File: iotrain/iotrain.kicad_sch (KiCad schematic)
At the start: 69 parts, among them J1 12V, J10 X2, J11 SCL, J12 SDA, J13 GND, J14 3V3, J15 GND, J16 USB_B_Micro, J2 PROG ESP, J3 AC1, J4 AC1, J5 LSP, J6 LSP, J7 M1, J8 M2, J9 X1, Q1 TPM2008 EP3-A, Q2 TPM2008 EP3-A, SW1 Reset, SW2 Boot, U2 MAX98357A_WLP_Package, U3 TPS82130, U4 ESP32-C6FH4, U6 IPS_160_40_10P, U7 DRV8876RGT, Y1 40MHz

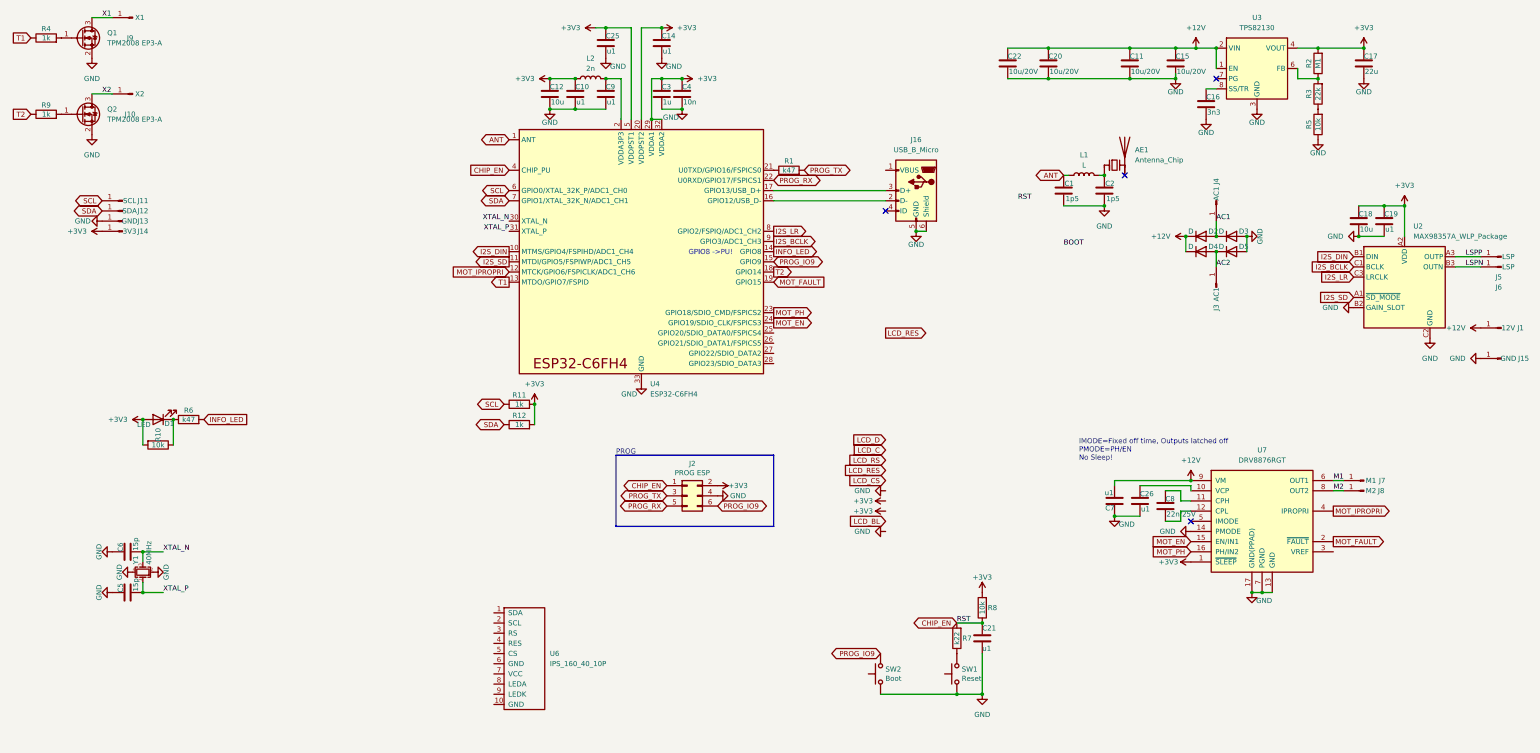
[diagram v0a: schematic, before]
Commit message: Beautified
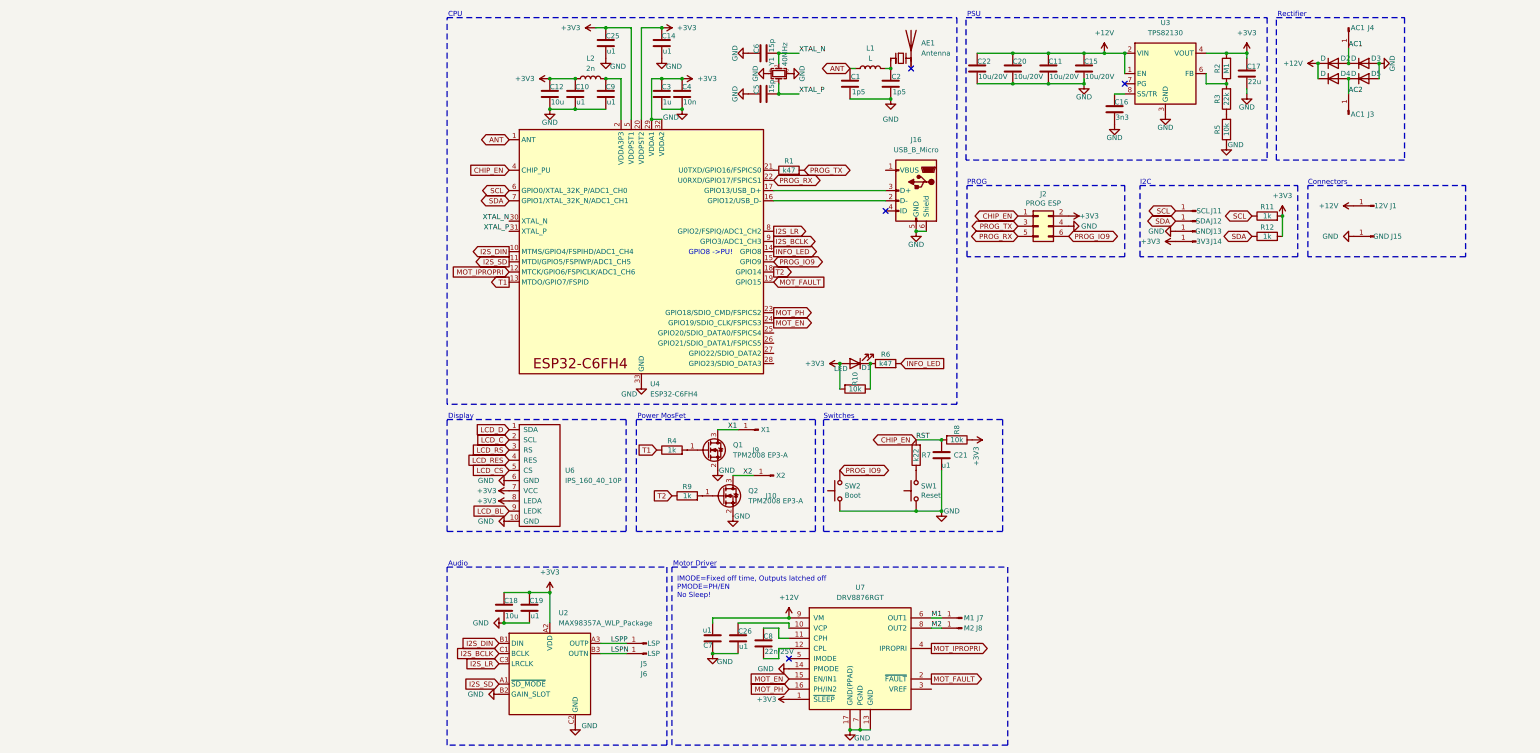
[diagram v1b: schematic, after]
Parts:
- AE1: value Antenna_Chip -> Antenna
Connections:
- net +3V3: now also R8.1, U6.7 (VCC), U6.8 (LEDA); no longer R8.2
- net CHIP_EN: now also R8.2; no longer R8.1
- net GND: now also U6.10 (GND), U6.6 (GND)
- net LCD_BL: now also U6.9 (LEDK)
- net LCD_C: now also U6.2 (SCL)
- net LCD_CS: now also U6.5 (CS)
- net LCD_D: now also U6.1 (SDA)
- net LCD_RES: now also U6.4 (RES)
- net LCD_RS: now also U6.3 (RS)
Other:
- note added: "Audio"
- note added: "CPU"
- note added: "Connectors"
- note added: "Display"
- note added: "I2C"
- note added: "Motor Driver"
- note added: "PSU"
- note added: "Power MosFet"
- note added: "Rectifier"
- note added: "Switches"
- moved on the sheet: AE1, C1, C11, C15, C16, C17, C18, C19, C2, C20, C21, C22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
